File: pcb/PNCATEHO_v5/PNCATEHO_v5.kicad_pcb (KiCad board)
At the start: 2 copper layers, 94.6 x 55 mm, 27 parts, among them J1 TestPoint_2Pole, SW1 SW_PUSH, SW10 SW_PUSH, SW2 SW_PUSH, SW3 SW_PUSH, SW4 SW_PUSH, SW5 SW_PUSH, SW6 SW_PUSH, SW7 SW_PUSH, SW8 SW_PUSH, SW9 SW_PUSH, U1 ProMicro_r

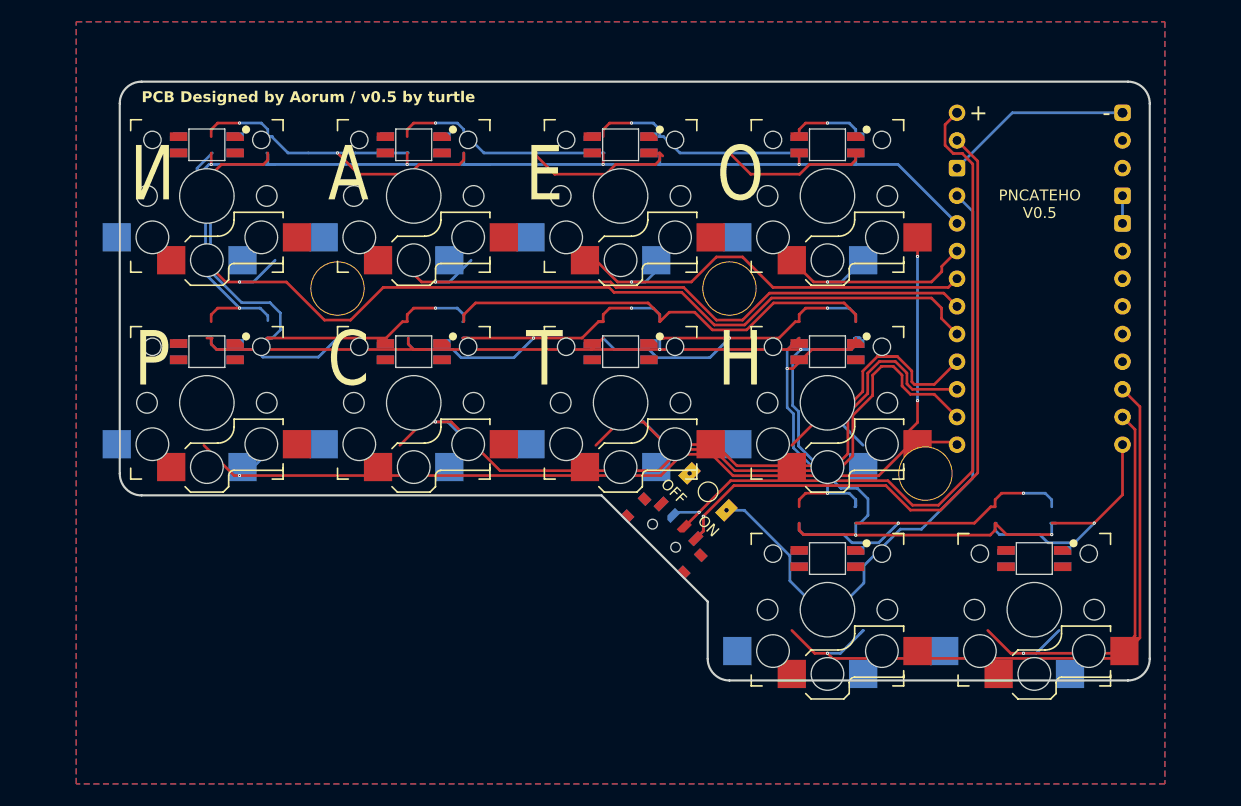
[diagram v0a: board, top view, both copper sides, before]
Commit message: Basic layout
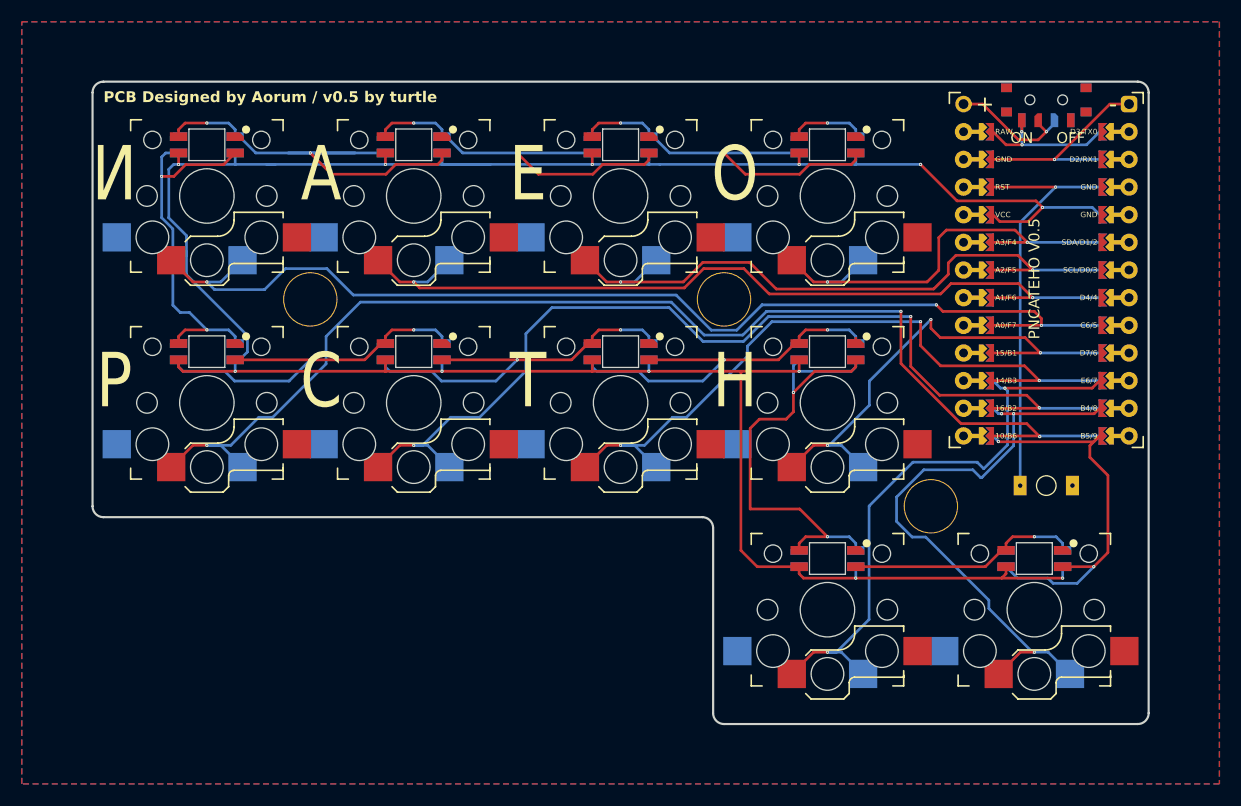
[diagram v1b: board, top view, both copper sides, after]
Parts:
- moved PSW1 55.5 mm to (114.1, 25.9), turned to 0 degrees
- moved RSW1 31.1 mm to (114.1, 62.6), turned to 0 degrees
- moved H3 3.04 mm to (103.5, 64.5)
- moved H1 2.69 mm to (46.5, 45.5)
- moved H2 1.12 mm to (84.5, 45.5)
- moved J1 1.00 mm to (114.1, 42.8)
- moved U1 1.00 mm to (114.1, 42.8)
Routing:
- net GND: track 63.3 -> 1.43 mm, vias 2 -> 0
- net Net-(PSW1-B): track 67.9 -> 12.0 mm
- net VBAT: track 64.7 -> 14.1 mm, vias 1 -> 2
- net Net-(LED3-DOUT): track 0.00 -> 35.5 mm, vias 0 -> 2
- net R2C1: track 77.8 -> 111.7 mm, vias 1 -> 3
- net R2C2: track 69.4 -> 91.2 mm, vias 1 -> 3
- net reset: track 59.7 -> 38.6 mm, vias 0 -> 1
- net R1C3: track 40.6 -> 60.1 mm, vias 1 -> 2
- net R1C1: track 81.2 -> 100.2 mm, vias 1 -> 3
- net R1C4: track 21.6 -> 40.6 mm, vias 1 -> 2
- net R1C2: track 59.1 -> 77.7 mm, vias 1 -> 2
- net R2C3: track 48.8 -> 66.4 mm, vias 1 -> 3
- net R2C4: track 28.3 -> 45.4 mm, vias 1 -> 3
- net R3C5: track 39.8 -> 55.0 mm, vias 1 -> 3
- net LED: track 23.2 -> 36.1 mm, vias 1 -> 2
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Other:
- board size 94.6 x 55 mm -> 97 x 59 mm
